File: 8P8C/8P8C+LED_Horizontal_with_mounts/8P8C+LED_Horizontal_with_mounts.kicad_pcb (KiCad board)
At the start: 2 copper layers, 30.6 x 25.4 mm, 6 parts, among them J1 8P8C_LED_Shielded, J2 Conn_01x06, J3 Conn_01x06

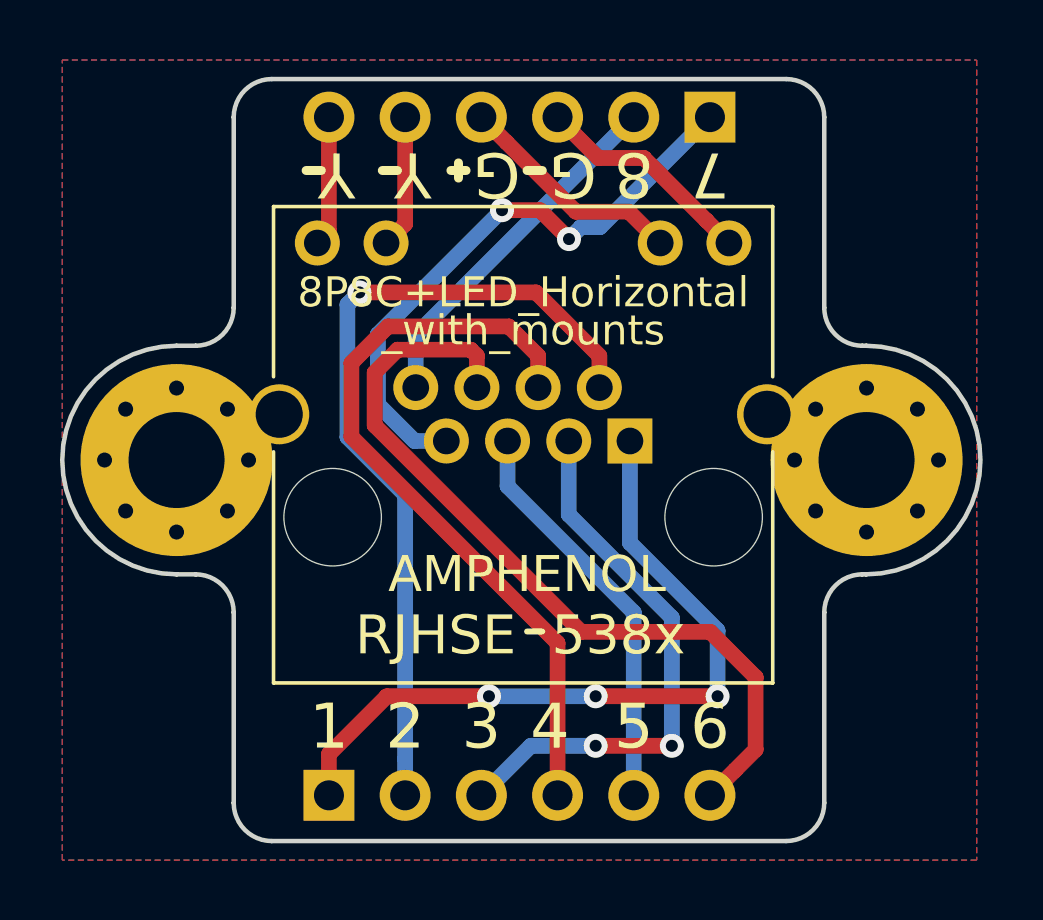
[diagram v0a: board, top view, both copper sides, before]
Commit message: Re-align pins
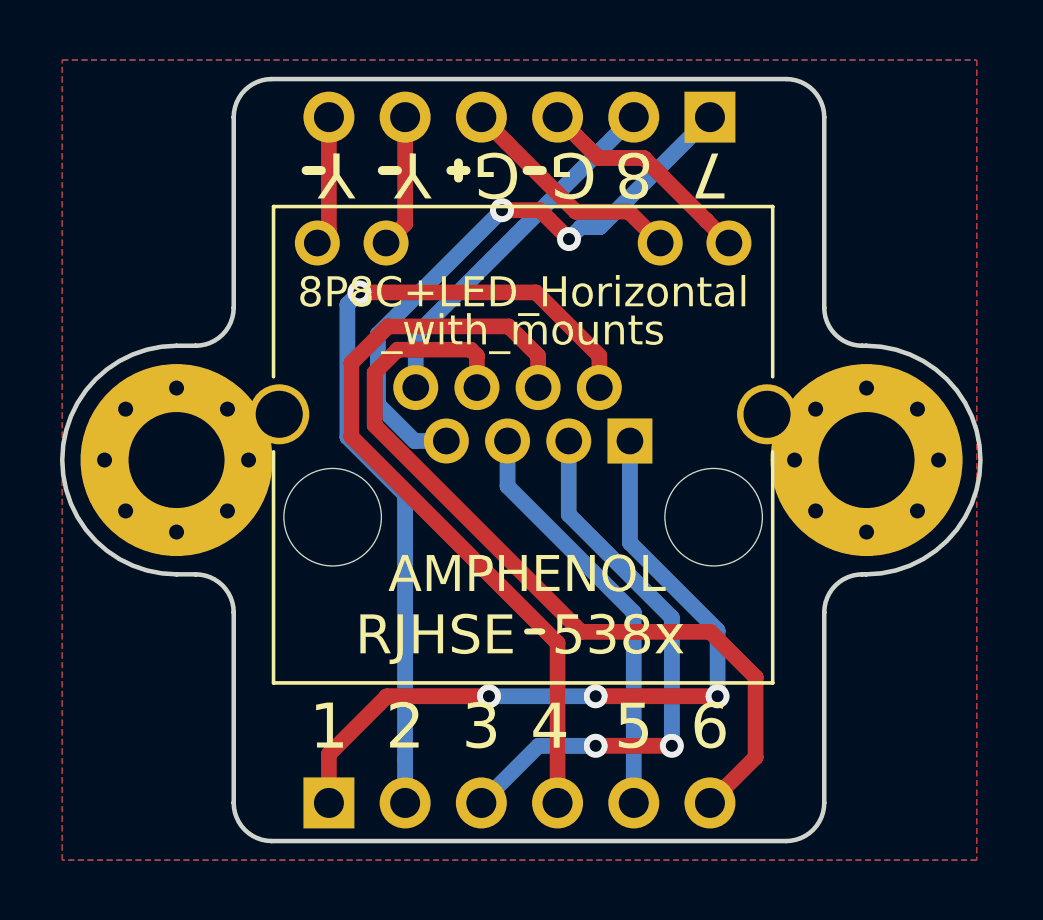
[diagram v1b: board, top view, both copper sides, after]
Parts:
- moved J2 0.25 mm to (134.6, 116.8)
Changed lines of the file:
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@@
     (thickness 1.6)
     (drawings 50)
-    (tracks 75)
+    (tracks 74)
     (zones 0)
     (modules 6)
@@
     (34 B.Paste user)
     (35 F.Paste user)
-    (36 B.SilkS user)
-    (37 F.SilkS user)
+    (36 B.SilkS user hide)
+    (37 F.SilkS user hide)
     (38 B.Mask user)
     (39 F.Mask user)
@@
   )
   (module Connector_PinHeader_2.54mm:PinHeader_1x06_P2.54mm_Vertical (layer B.Cu)
-    (at 134.62 116.586 270)
+    (at 134.62 116.84 270)
     (descr "Through hole straight pin header, 1x06, 2.54mm pitch, single row")
     (tags "Through hole pin header THT 1x06 2.54mm single row")
@@
   (segment (start 137.513 101.247) (end 144.78 93.98) (width 0.525) (layer B.Cu) (net 6))
   (segment (start 137.513 102.995) (end 137.513 101.247) (width 0.525) (layer B.Cu) (net 6))
-  (segment (start 148.169999 115.736001) (end 147.32 116.586) (width 0.525) (layer F.Cu) (net 7))
   (segment (start 147.33301 111.13801) (end 148.844 112.649) (width 0.525) (layer F.Cu) (net 7))
   (segment (start 143.01501 111.13801) (end 147.33301 111.13801) (width 0.525) (layer F.Cu) (net 7))
   (segment (start 143.01501 111.125512) (end 143.01501 111.13801) (width 0.525) (layer F.Cu) (net 7))
-  (segment (start 148.844 112.649) (end 148.844 115.062) (width 0.525) (layer F.Cu) (net 7))
   (segment (start 139.553 101.93434) (end 139.351159 101.732499) (width 0.525) (layer F.Cu) (net 7))
   (segment (start 139.553 102.995) (end 139.553 101.93434) (width 0.525) (layer F.Cu) (net 7))
   (segment (start 139.351159 101.732499) (end 136.906999 101.732499) (width 0.525) (layer F.Cu) (net 7))
   (segment (start 136.906999 101.732499) (end 136.144 102.495498) (width 0.525) (layer F.Cu) (net 7))
-  (segment (start 148.844 115.062) (end 148.169999 115.736001) (width 0.525) (layer F.Cu) (net 7))
   (segment (start 136.144 102.495498) (end 136.144 104.254502) (width 0.525) (layer F.Cu) (net 7))
   (segment (start 136.144 104.254502) (end 143.01501 111.125512) (width 0.525) (layer F.Cu) (net 7))
+  (segment (start 148.844 115.316) (end 147.32 116.84) (width 0.525) (layer F.Cu) (net 7))
+  (segment (start 148.844 112.649) (end 148.844 115.316) (width 0.525) (layer F.Cu) (net 7))
   (segment (start 135.36899 102.174479) (end 135.36899 104.63499) (width 0.525) (layer F.Cu) (net 8))
   (segment (start 136.58598 100.957489) (end 135.36899 102.174479) (width 0.525) (layer F.Cu) (net 8))
@@
   (via (at 143.51 114.935) (size 0.8) (drill 0.4) (layers F.Cu B.Cu) (net 12))
   (segment (start 146.05 114.935) (end 143.51 114.935) (width 0.525) (layer F.Cu) (net 12))
-  (segment (start 141.351 114.935) (end 139.7 116.586) (width 0.525) (layer B.Cu) (net 12))
-  (segment (start 143.51 114.935) (end 141.351 114.935) (width 0.525) (layer B.Cu) (net 12))
+  (segment (start 141.605 114.935) (end 139.7 116.84) (width 0.525) (layer B.Cu) (net 12))
+  (segment (start 143.51 114.935) (end 141.605 114.935) (width 0.525) (layer B.Cu) (net 12))
   (via (at 147.574 113.284) (size 0.8) (drill 0.4) (layers F.Cu B.Cu) (net 13))
   (segment (start 147.574 111.091948) (end 147.574 113.284) (width 0.525) (layer B.Cu) (net 13))
